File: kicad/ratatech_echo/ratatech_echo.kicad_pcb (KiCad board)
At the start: 2 copper layers, 99.8 x 90 mm, 108 parts, among them J1 AudioJack2, J2 Conn_01x02, J3 Conn_01x02, J4 AudioJack2, J5 Barrel_Jack_Switch, Q1 2N3904, Q2 2N3906, Q3 2N3904, Q4 2N3906, SW1 SW_SPDT, SW2 SW_SPST, U1 NE5532, U2 NE5532, U3 PT2399, U4 LT1054xSOIC16, U5 LM7812_TO220, U6 LM7912_TO220

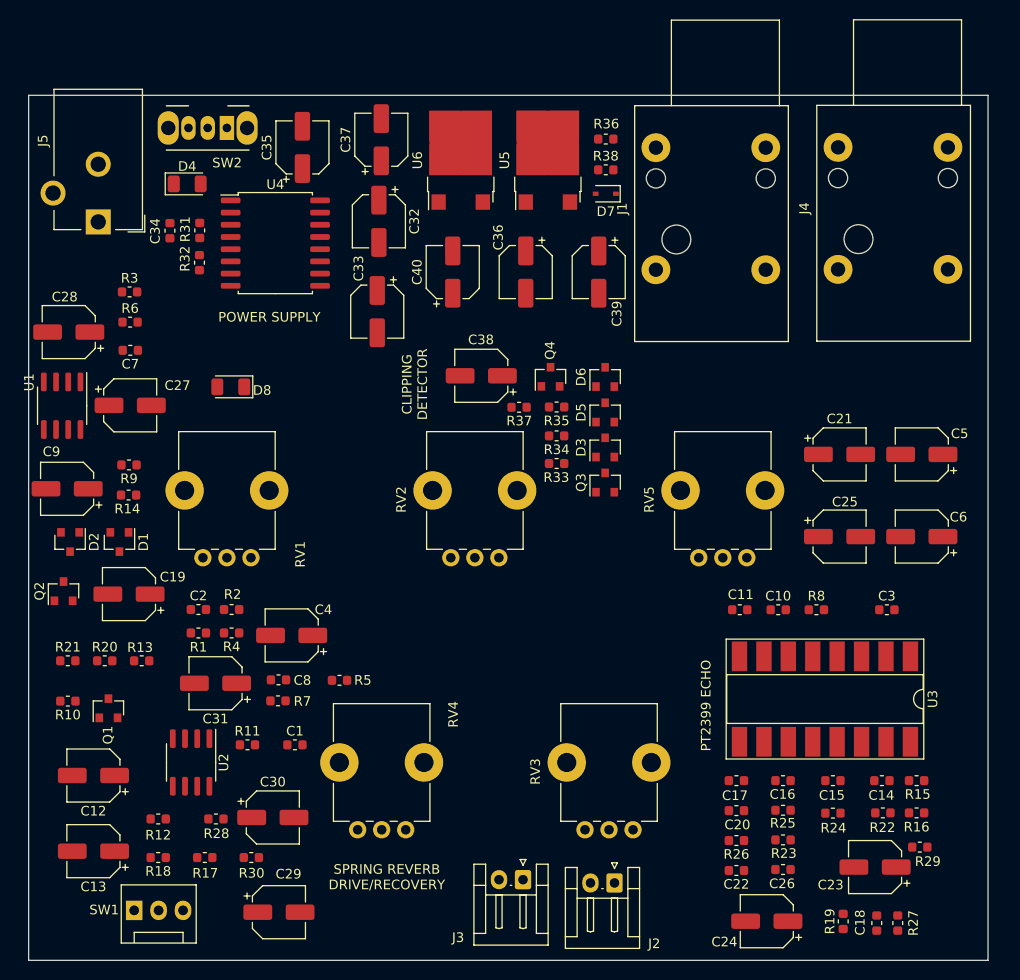
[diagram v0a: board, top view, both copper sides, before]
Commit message: Routing full done first try
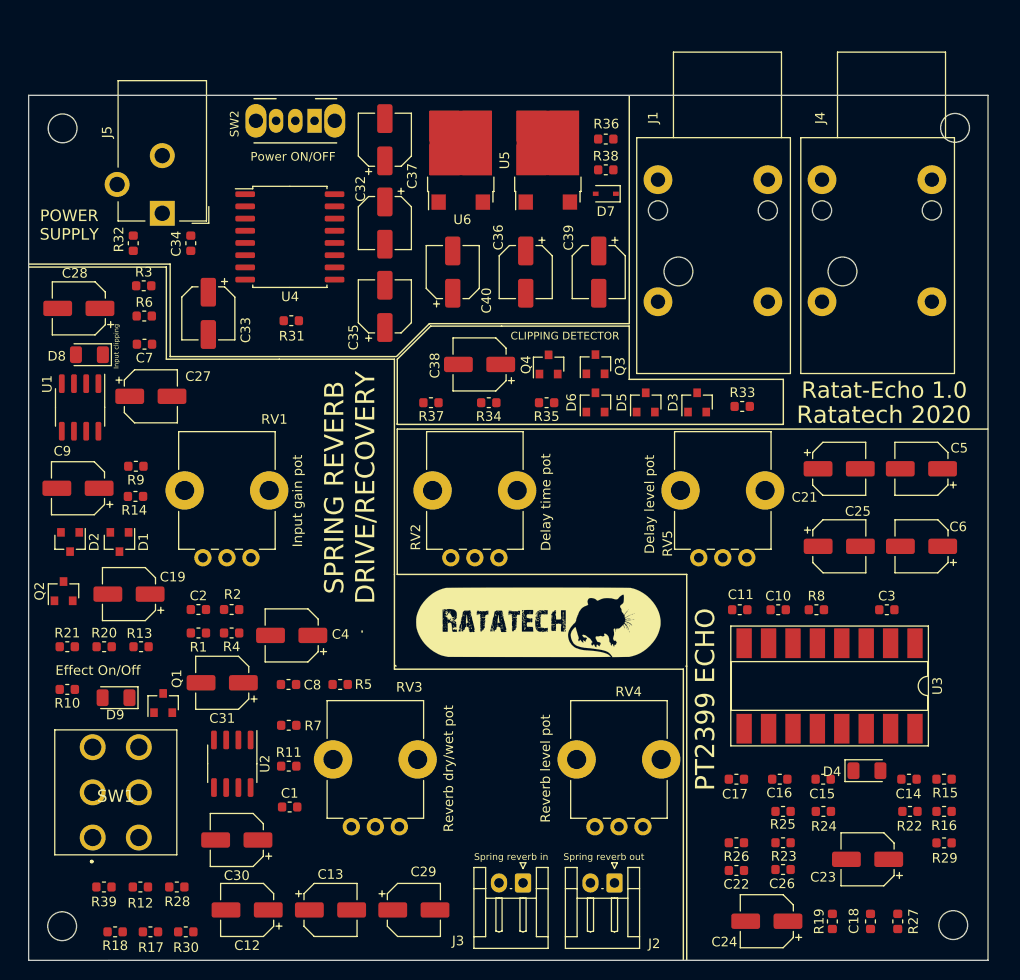
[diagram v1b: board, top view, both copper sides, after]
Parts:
- removed C20: 560uF, Capacitor_SMD:C_0603_1608Metric
- added D9: LED, LED_SMD:LED_1206_3216Metric, F.Cu at (106.7, 86.2)
- added G***: LOGO, imgs:ratatech_bitmap, F.Cu at (150.7, 78.3)
- added R39: 470, Resistor_SMD:R_0603_1608Metric, F.Cu at (105.5, 105.9)
- added REF**: MountingHole_3mm, MountingHole:MountingHole_3mm, F.Cu at (101.1, 27.0)
- added REF**: MountingHole_3mm, MountingHole:MountingHole_3mm, F.Cu at (101.1, 110.0)
- added REF**: MountingHole_3mm, MountingHole:MountingHole_3mm, F.Cu at (194.0, 26.9)
- added REF**: MountingHole_3mm, MountingHole:MountingHole_3mm, F.Cu at (193.8, 109.9)
- SW1: value SW_SPDT -> SW_DPDT_x2; footprint Connector:FanPinHeader_1x03_P2.54mm_Vertical -> M2028B2B1W03:M2028B2B1W03
- moved D4 93.4 mm to (184.8, 93.8)
- moved C13 25.4 mm to (129.0, 108.3), turned to 0 degrees
- moved RV4 24.7 mm to (159.0, 92.0)
- moved RV3 24.3 mm to (133.6, 92.0)
- moved C12 21.2 mm to (120.3, 108.3)
- moved R33 20.2 mm to (171.9, 55.9), turned to 180 degrees
- moved C35 18.6 mm to (134.7, 45.5)
- moved C33 17.6 mm to (116.3, 46.2)
- moved D8 15.1 mm to (103.9, 50.5)
- moved C29 14.0 mm to (137.7, 108.3)
- moved R31 13.4 mm to (124.9, 47.0), turned to 0 degrees
- moved SW1 12.8 mm to (106.8, 95.7)
- moved Q3 12.4 mm to (156.6, 51.5)
- moved D3 10.7 mm to (167.2, 55.5)
- moved R30 10.3 mm to (114.0, 110.6)
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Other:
- board text added: "Delay level pot"
- board text added: "Delay time pot"
- board text added: "Effect On/Off"
- board text added: "Input clipping"
- board text added: "Input gain pot"
- board text added: "Power ON/OFF"
- board text added: "Ratat-Echo 1.0"
- board text added: "Ratatech 2020"
- board text added: "Reverb dry/wet pot"
- board text added: "Reverb level pot"
- board text added: "Spring reverb in"
- board text added: "Spring reverb out"
